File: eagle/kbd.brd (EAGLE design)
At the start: 41.1 x 72.1 mm, 29 parts, among them U1 STM32L011

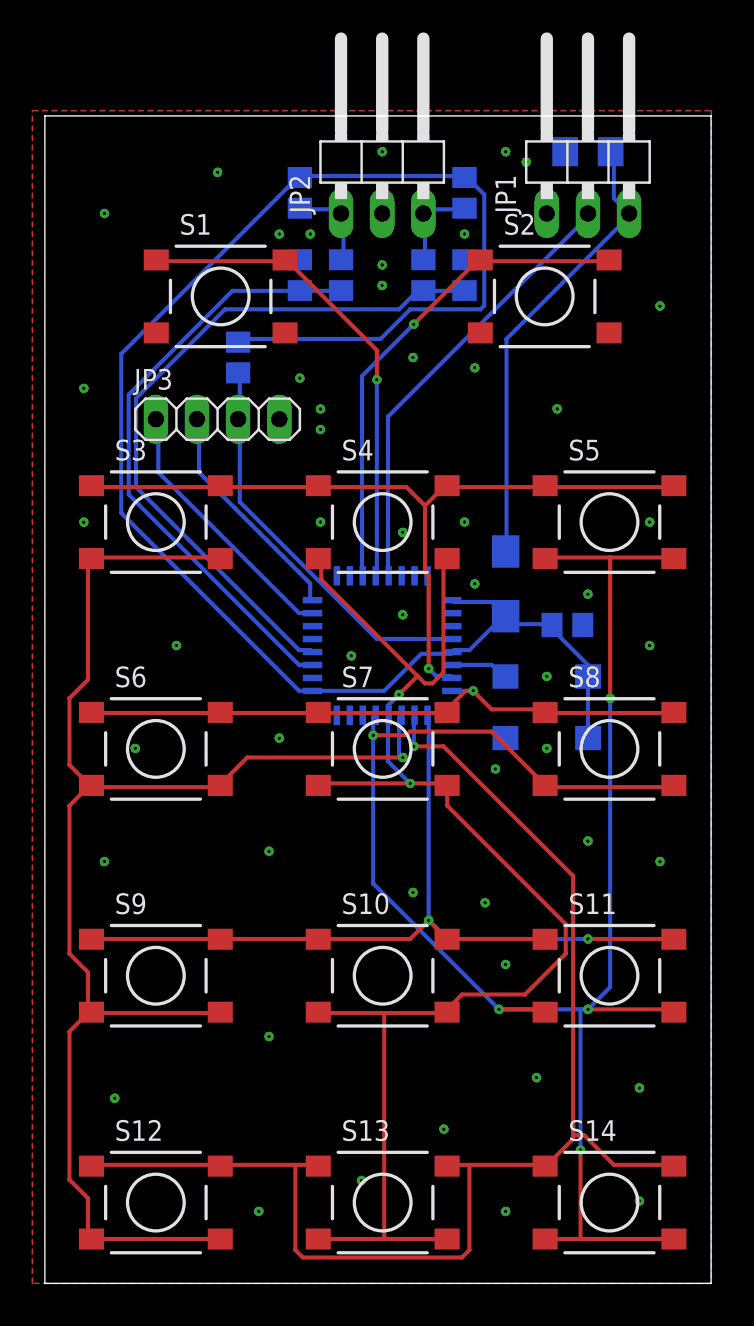
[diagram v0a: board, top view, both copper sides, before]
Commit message: Add files via upload
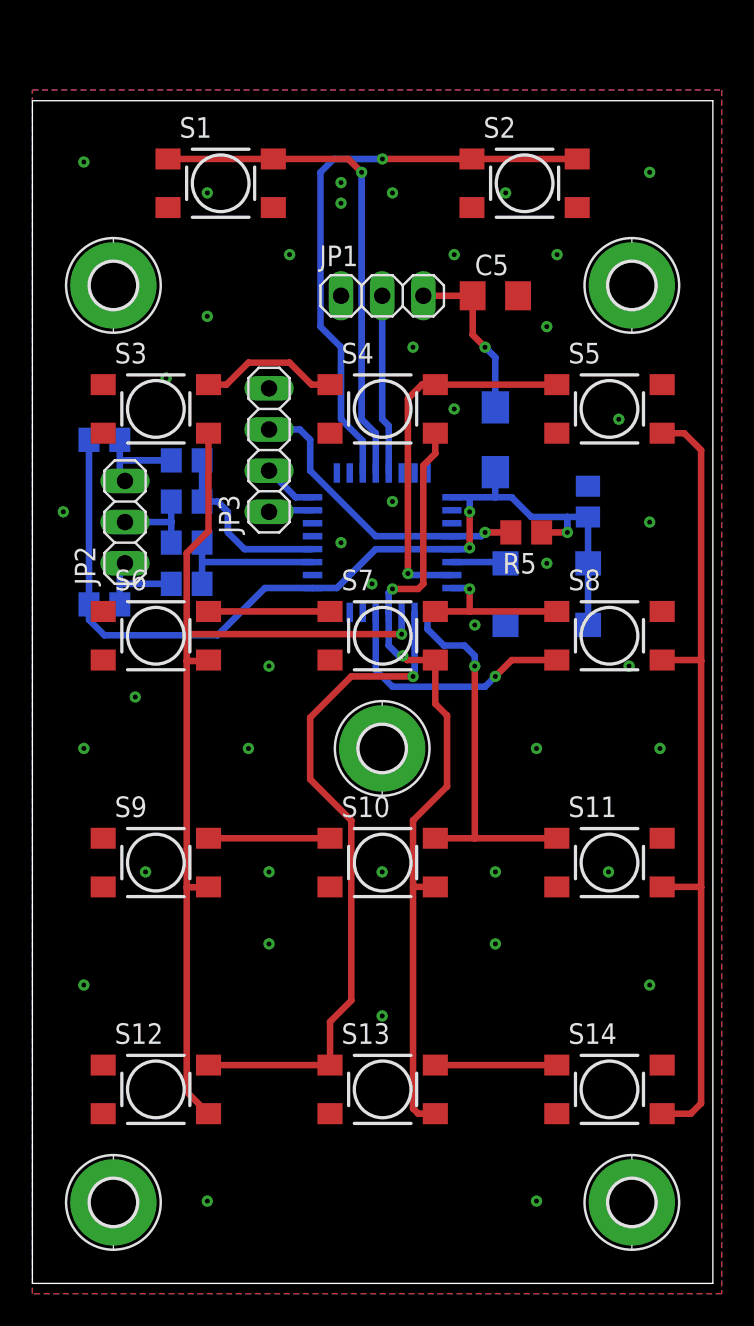
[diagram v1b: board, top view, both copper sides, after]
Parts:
- added H1, H2, H3, H4, H5: MOUNT-PAD-ROUND2.8, holes:2,8-PAD
- JP1, JP2: device pinhead:1X03/90 -> pinhead:1X03
- moved R2 28.1 mm to (4.45, 41.9), turned to 0 degrees
- moved JP2 27.8 mm to (5.71, 47.0), turned to 90 degrees
- moved R1 26.9 mm to (4.45, 52.1), turned to 0 degrees
- moved C4 22.1 mm to (9.53, 48.3), turned to 0 degrees
- moved R3 21.3 mm to (9.53, 43.2), turned to 180 degrees
- moved R5 20.8 mm to (30.5, 46.4), flipped to the top, turned to 180 degrees
- moved R4 18.5 mm to (9.53, 50.8), turned to 180 degrees
- moved C3 17.9 mm to (9.53, 45.7), turned to 0 degrees
- moved JP1 15.5 mm to (21.6, 61.0)
- moved C5 10.6 mm to (28.6, 61.0), flipped to the top
- moved L1 8.91 mm to (28.6, 52.1)
- moved C2 7.73 mm to (34.3, 48.3), turned to 90 degrees
- moved S2 7.09 mm to (30.4, 67.9)
- moved S10 6.99 mm to (21.6, 26.0)
- moved S11 6.99 mm to (35.6, 26.0)
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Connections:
- net GND: now also H1.B2,8, H2.B2,8, H3.B2,8, H4.B2,8, H5.B2,8
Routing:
- net C3: track 114.1 -> 66.5 mm, vias 5 -> 1
- net +3V3: track 105.3 -> 60.0 mm, vias 0 -> 3
- net C2: track 87.2 -> 50.2 mm
- net R4: track 82.7 -> 49.4 mm
- net ENC_A: track 43.8 -> 11.3 mm
- net C1: track 92.5 -> 60.5 mm
- net ENC_B: track 37.6 -> 9.38 mm
- net R3: track 57.3 -> 30.9 mm, vias 2 -> 1
- net R2: track 38.6 -> 17.5 mm
- net N$3: track 28.3 -> 10.5 mm, vias 0 -> 1
- net R1: track 49.2 -> 31.7 mm
- net TX: track 27.5 -> 11.1 mm
- net SWDIO: track 16.5 -> 2.78 mm
- net SWCLK: track 14.2 -> 3.37 mm
- net NRST: track 24.7 -> 18.9 mm, vias 0 -> 1
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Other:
- board size 41.1 x 72.1 mm -> 42 x 73 mm
- board text added: "A"
- board text added: "B"
- board text added: "B1"
- board text added: "B2"
- board text added: "ENCODER"
- board text added: "GND"
- board text added: "PWR"
- board text added: "SWD"
- board text added: "TX"
